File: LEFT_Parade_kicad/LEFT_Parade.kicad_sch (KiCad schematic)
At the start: 31 parts, among them SW1 RotaryEncoder_Switch, SW10 SW_Push_reverse, SW11 SW_Push_reverse, SW12 SW_Push_reverse, SW13 SW_Push_reverse, SW14 SW_Push_reverse, SW15 SW_Push_reverse, SW16 SW_Push_reverse, SW17 SW_Push_reverse, SW2 SW_Push, SW3 SW_Push, SW4 SW_Push, SW5 SW_Push, SW6 SW_Push, SW7 SW_Push, SW8 SW_Push, SW9 SW_Push, U1 SeeeduinoXIAO, U2 74LS139

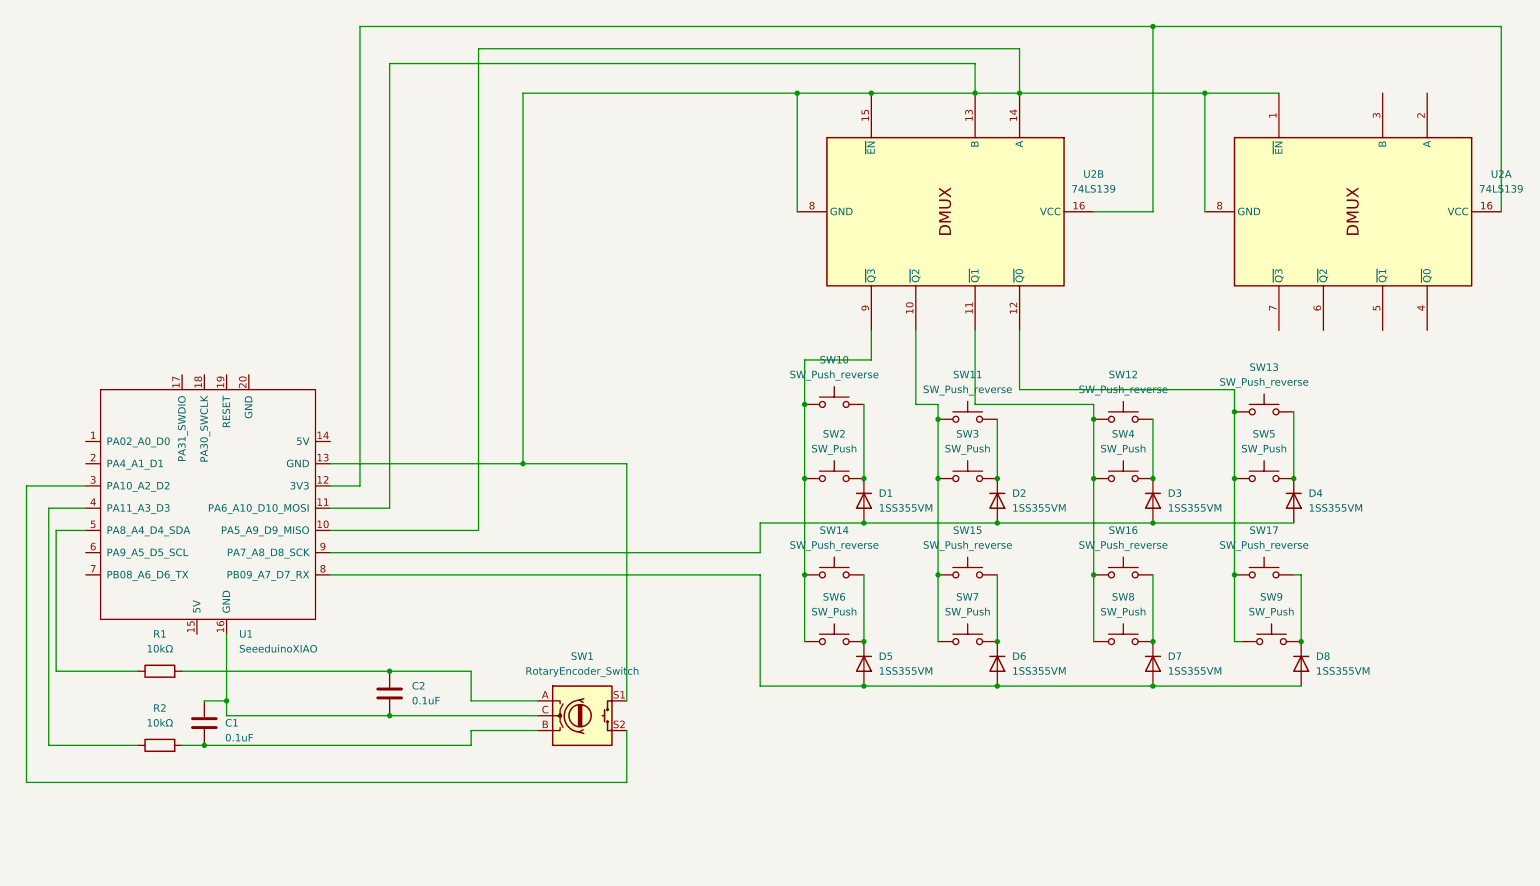
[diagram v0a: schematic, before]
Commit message: [Modify] thankyou...
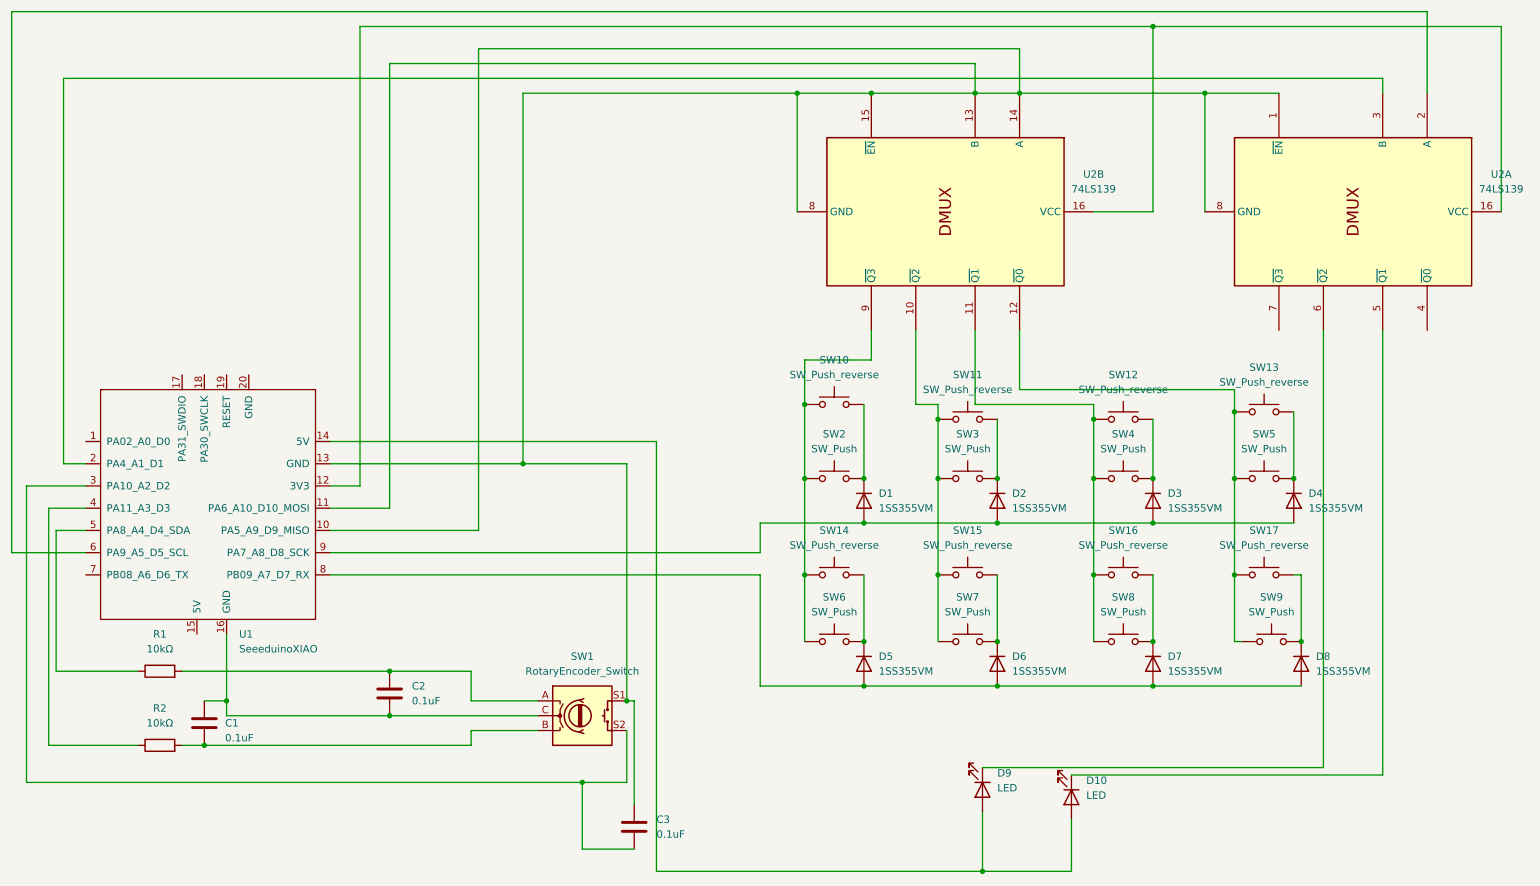
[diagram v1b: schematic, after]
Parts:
- added C3: 0.1uF, Capacitor_THT:C_Axial_L5.1mm_D3.1mm_P7.50mm_Horizontal, symbol Device:C
- added D10, D9: LED, LED_THT:LED_D3.0mm_Clear, symbol Device:LED
- SW10, SW11, SW12, SW13, SW14, SW15, SW16, SW17: footprint Button_Switch_Keyboard:SW_Cherry_MX_1.25u_PCB -> esp32_xiao:SW_Cherry_MX_1.00u_PCB_reverse
- SW2, SW3, SW4, SW5, SW6, SW7, SW8, SW9: footprint Button_Switch_Keyboard:SW_Cherry_MX_1.25u_PCB -> Button_Switch_Keyboard:SW_Cherry_MX_1.00u_PCB
- U1: footprint (none) -> esp32_xiao:ESP32C3_Footprint
- U2: footprint (none) -> Package_DIP:CERDIP-16_W7.62mm_SideBrazed
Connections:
- net at SW1.S1, U1.10 (PA5_A9_D9_MISO), U1.11 (PA6_A10_D10_MOSI)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: now also C3.1
- net at U2.2 (A): now also U1.6 (PA9_A5_D5_SCL)
- net at U2.3 (B): now also U1.2 (PA4_A1_D1)
- net at U2.5 (~{Q1}): now also D10.1 (K)
- net at U2.6 (~{Q2}): now also D9.1 (K)
- net at U1.14 (5V): now also D10.2 (A), D9.2 (A)
- net at SW1.S2, U1.3 (PA10_A2_D2): now also C3.2
